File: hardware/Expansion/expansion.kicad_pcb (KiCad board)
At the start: 2 copper layers, 91.7 x 48 mm, 27 parts, among them J1 VID, J2 PPI, J3 PPO, P1 EXI, P2 EXO, U1 74LS138, U2 74LS00, U3 74LS123, U4 74LS20, U5 74LS175, U6 74LS245

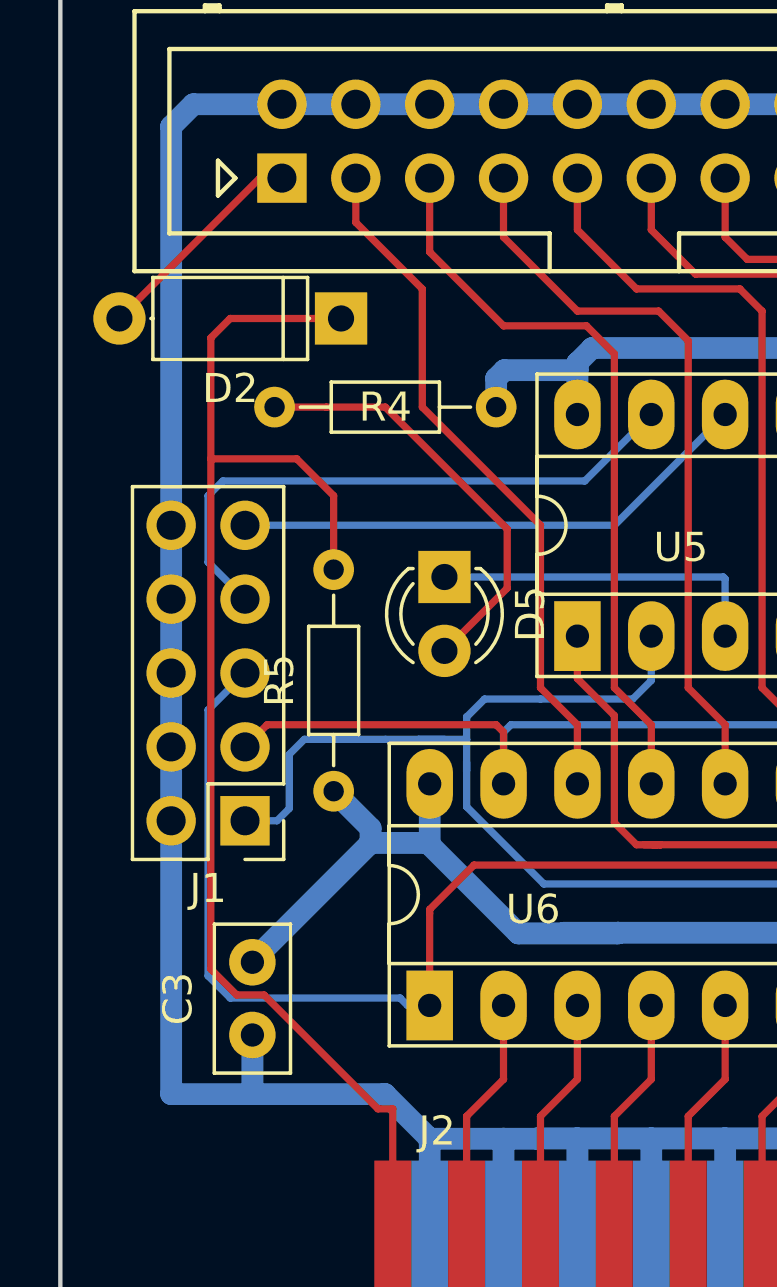
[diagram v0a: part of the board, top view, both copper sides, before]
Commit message: Revert "update:expansion"
This reverts commit fc7daa09fcab310e52193976a9df76314ecc8e0b.
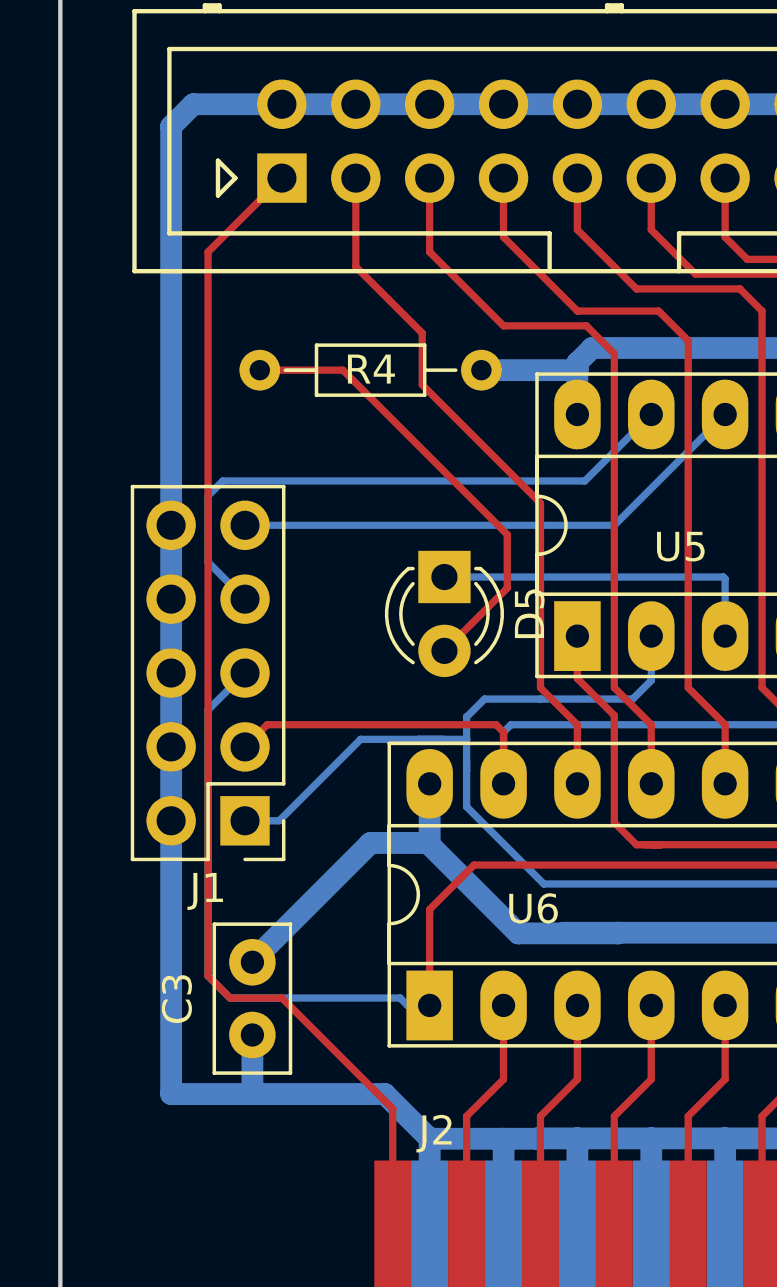
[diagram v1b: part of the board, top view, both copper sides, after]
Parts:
- removed D2: D, Diodes_THT:D_A-405_P7.62mm_Horizontal
- removed R5: 470, Resistors_THT:R_Axial_DIN0204_L3.6mm_D1.6mm_P7.62mm_Horizontal
- moved R4 1.37 mm to (38.6, 40.1)
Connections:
- J2 pad 1: /STBI -> /STB
- J3 pad 1: /STBO -> /STB
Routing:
- net /STBI: track 46.3 -> 0.00 mm
- net /STB: track 0.00 -> 41.0 mm
- net /STBO: track 7.59 -> 0.00 mm
- net VCC: track 259.0 -> 256.1 mm
- net /EMAP: track 107.4 -> 106.3 mm
- net Net-(D5-Pad2): track 14.8 -> 15.7 mm

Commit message: revert:expansion
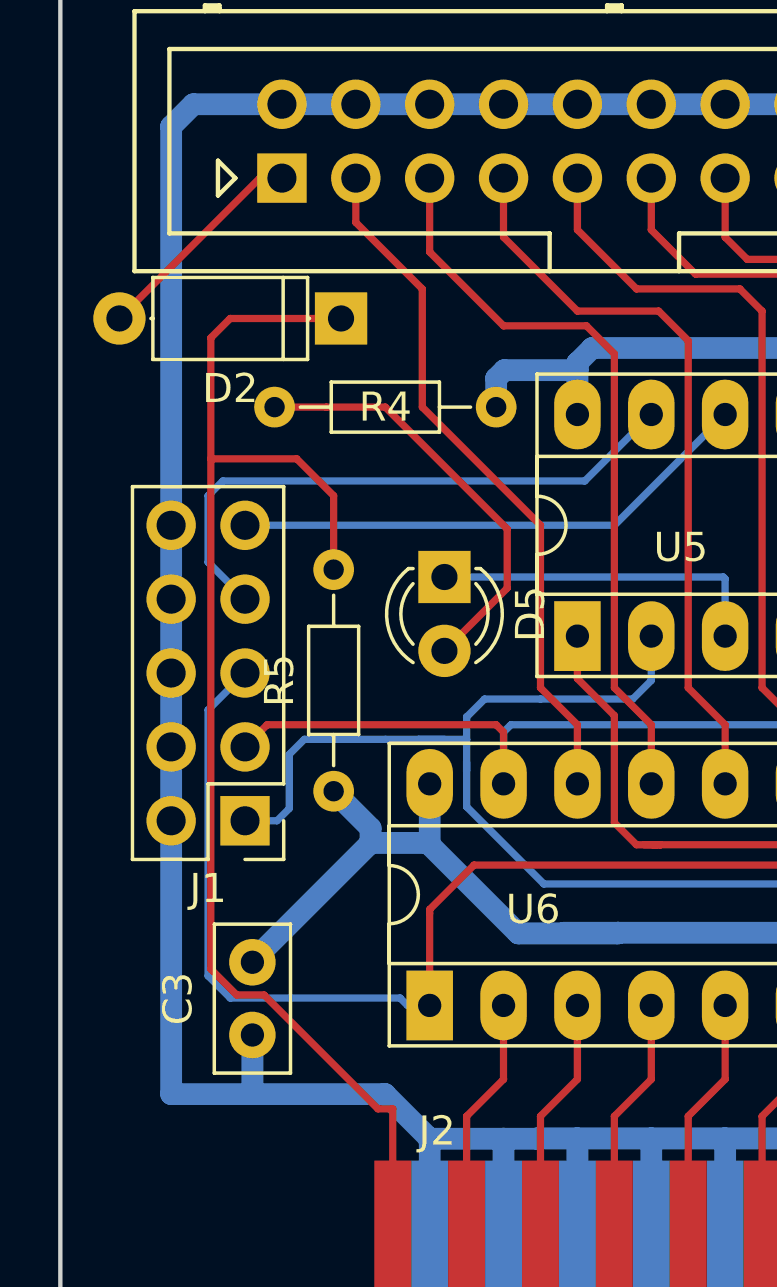
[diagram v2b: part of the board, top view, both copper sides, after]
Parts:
- added D2: D, Diodes_THT:D_A-405_P7.62mm_Horizontal, F.Cu at (33.8, 38.4)
- added R5: 470, Resistors_THT:R_Axial_DIN0204_L3.6mm_D1.6mm_P7.62mm_Horizontal, F.Cu at (33.5, 54.6)
- moved R4 1.37 mm to (39.1, 41.4)
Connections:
- J2 pad 1: /STB -> /STBI
- J3 pad 1: /STB -> /STBO
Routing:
- net /STBI: track 0.00 -> 46.3 mm
- net /STB: track 41.0 -> 0.00 mm
- net /STBO: track 0.00 -> 7.59 mm
- net VCC: track 256.1 -> 259.0 mm
- net /EMAP: track 106.3 -> 107.4 mm
- net Net-(D5-Pad2): track 15.7 -> 14.8 mm

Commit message: .
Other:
- net class Default removed
- net class Power removed
